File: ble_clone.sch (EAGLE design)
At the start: 24 parts, among them IC1 PIC24FV16KM202, IC2 3.3 vreg

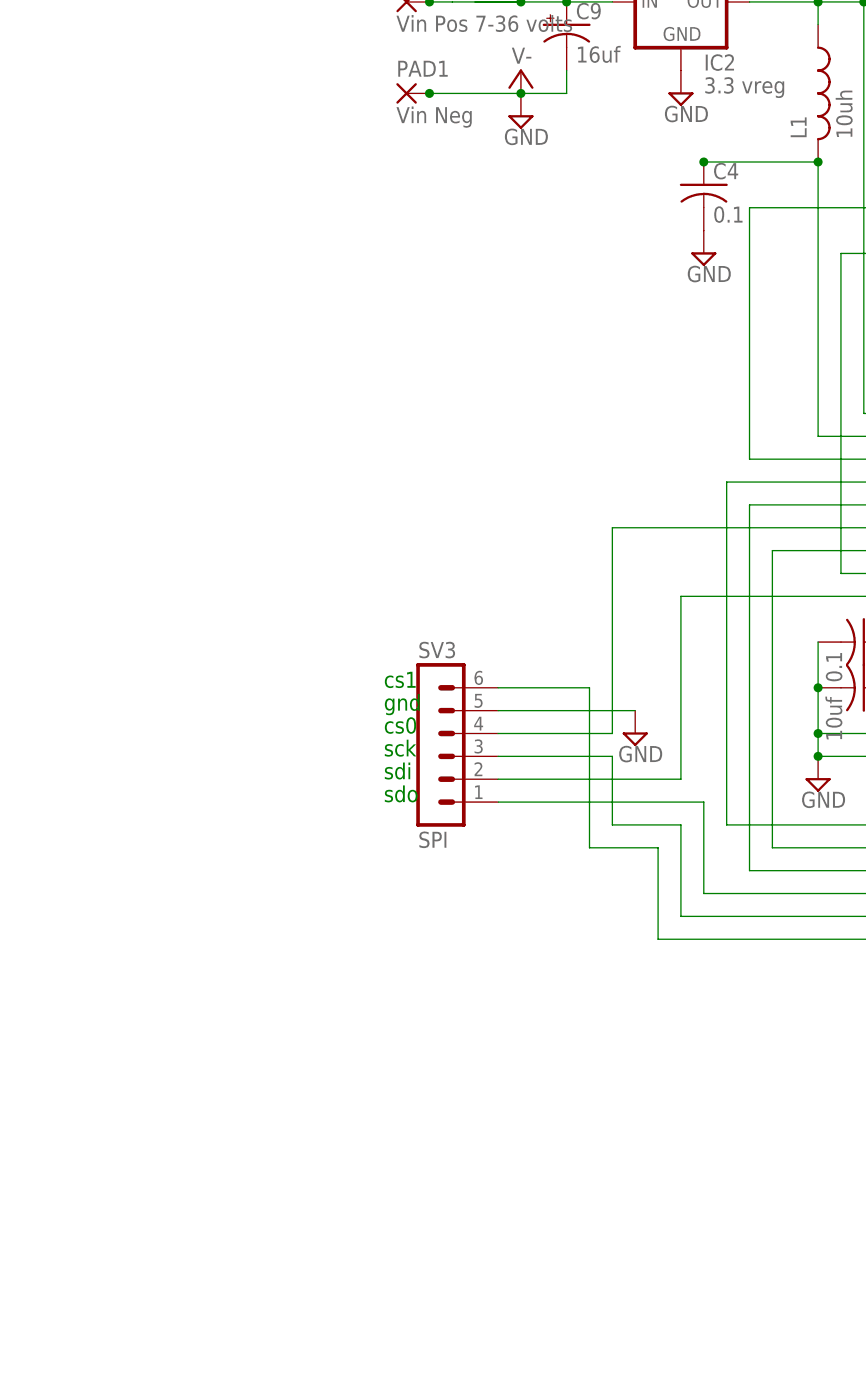
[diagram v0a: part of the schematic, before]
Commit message: updates
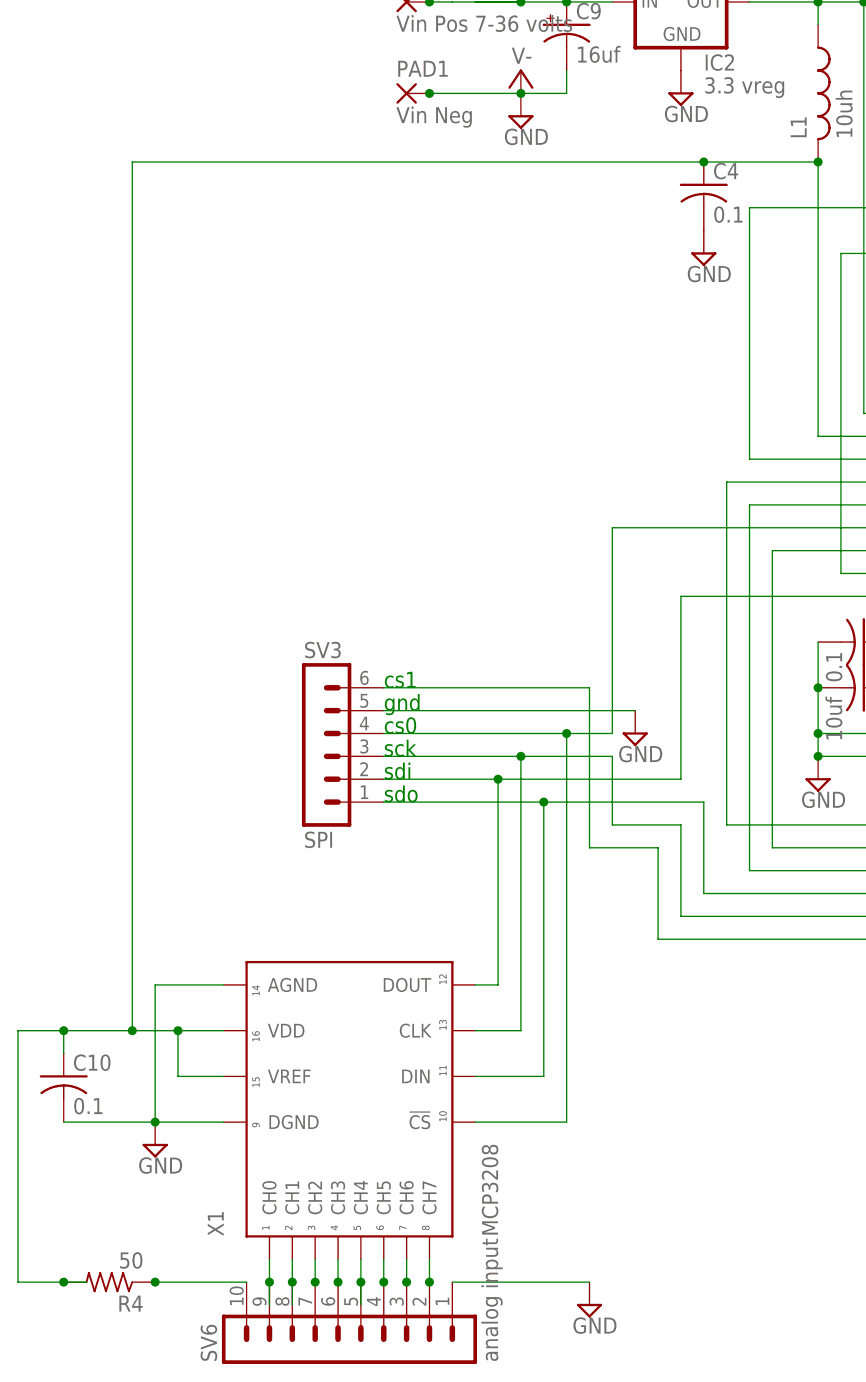
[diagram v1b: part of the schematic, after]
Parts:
- added C10: 0.1, resistor:C-US025-024X044
- added R4: 50, resistor:R-US_0204/2V
- added SV6: analog input, con-lstb:MA10-1
- added X1: MCP3208, Microchip:21298EDIP
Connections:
- new net N$34: SV6.2, X1.CH7
- new net N$35: SV6.3, X1.CH6
- new net N$36: SV6.4, X1.CH5
- new net N$37: SV6.5, X1.CH4
- new net N$38: SV6.6, X1.CH3
- new net N$39: SV6.7, X1.CH2
- new net N$40: SV6.8, X1.CH1
- new net N$41: SV6.9, X1.CH0
- new net N$43: R4.1, SV6.10
- net GND: now also C10.2, SV6.1, X1.AGND, X1.DGND
- net N$16: now also C10.1, R4.2, X1.VDD, X1.VREF
- net N$18: now also X1.!CS
- net N$19: now also X1.DOUT
- net N$20: now also X1.DIN
- net N$21: now also X1.CLK
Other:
- moved on the sheet: SV3
